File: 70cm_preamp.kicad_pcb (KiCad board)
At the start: 2 copper layers, 33 x 13.2 mm, 10 parts, among them J1 RF_IN, J2 RF_OUT, U1 SF2446E, U2 PGA-103+

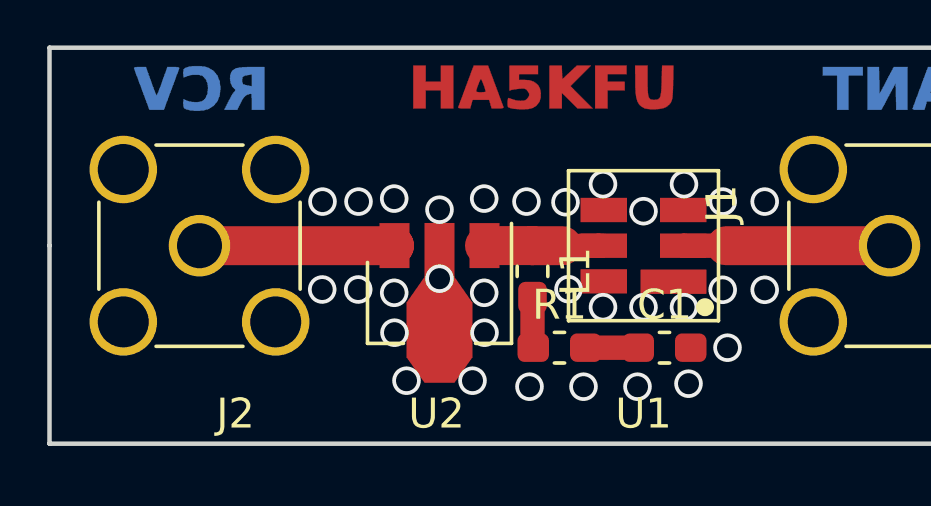
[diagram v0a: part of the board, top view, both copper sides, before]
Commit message: 0805 RLC
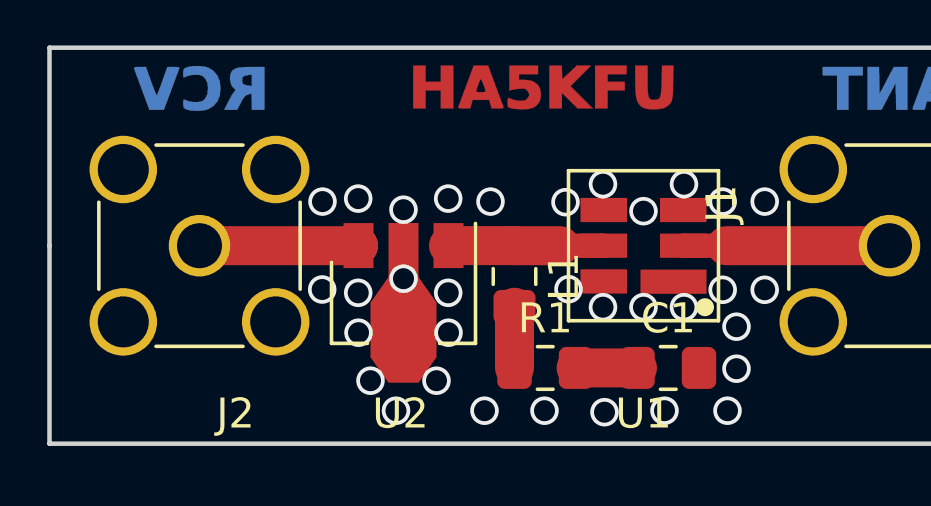
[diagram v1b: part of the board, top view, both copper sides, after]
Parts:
- C1: footprint 70cm_preamp:C_0603_1608Metric_Pad1.05x0.95mm_HandSolder -> 70cm_preamp:C_0805_2012Metric_Pad1.15x1.40mm_HandSolder
- L1: footprint 70cm_preamp:L_0603_1608Metric_Pad1.05x0.95mm_HandSolder -> 70cm_preamp:L_0805_2012Metric_Pad1.15x1.40mm_HandSolder
- R1: footprint 70cm_preamp:R_0603_1608Metric_Pad1.05x0.95mm_HandSolder -> 70cm_preamp:R_0805_2012Metric_Pad1.15x1.40mm_HandSolder
- moved U2 1.20 mm to (54.4, 38.3)
- moved R1 0.83 mm to (59.1, 40.9)
- moved C1 0.69 mm to (63.2, 40.9)
- moved L1 0.62 mm to (58.1, 37.8)
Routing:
- net Net-(L1-Pad1): track 3.38 -> 5.18 mm
- net Net-(J2-Pad1): track 6.50 -> 5.30 mm
- net GND: vias 32 -> 33

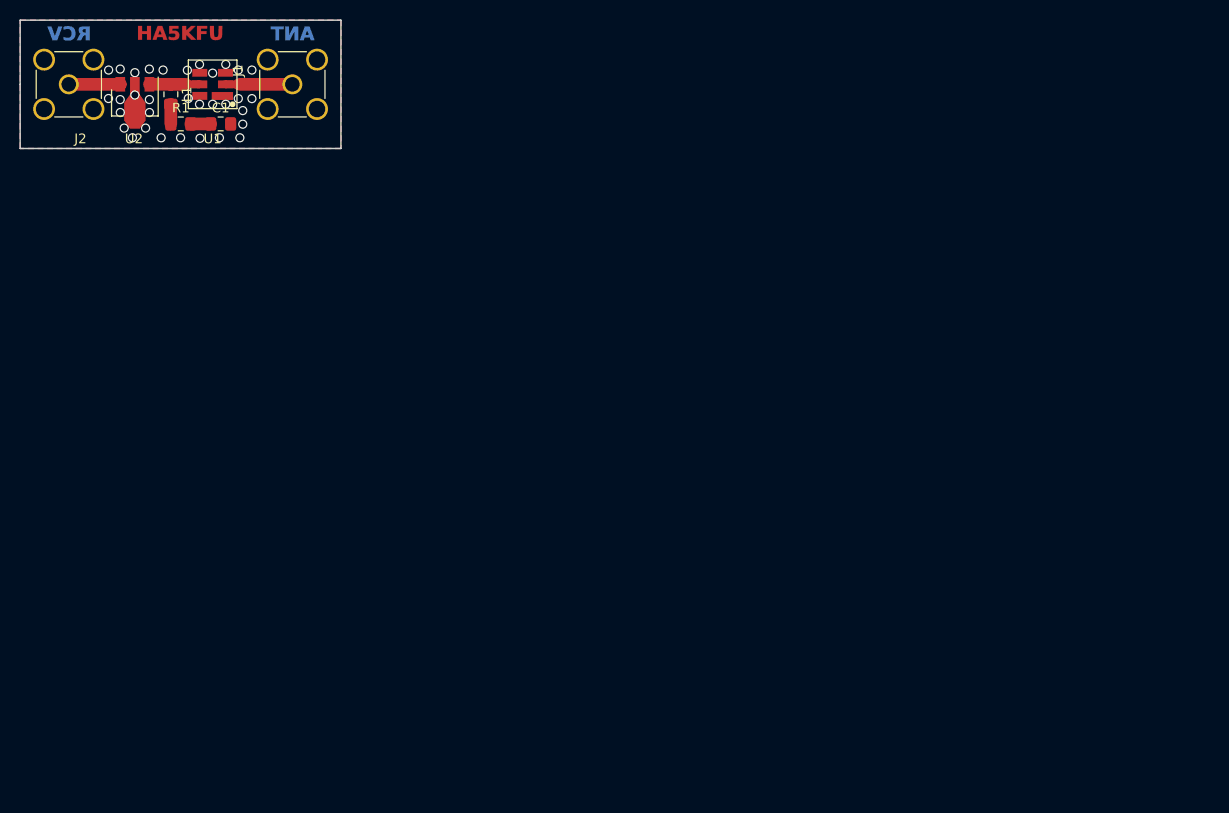
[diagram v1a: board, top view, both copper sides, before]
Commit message: Dokumentáció
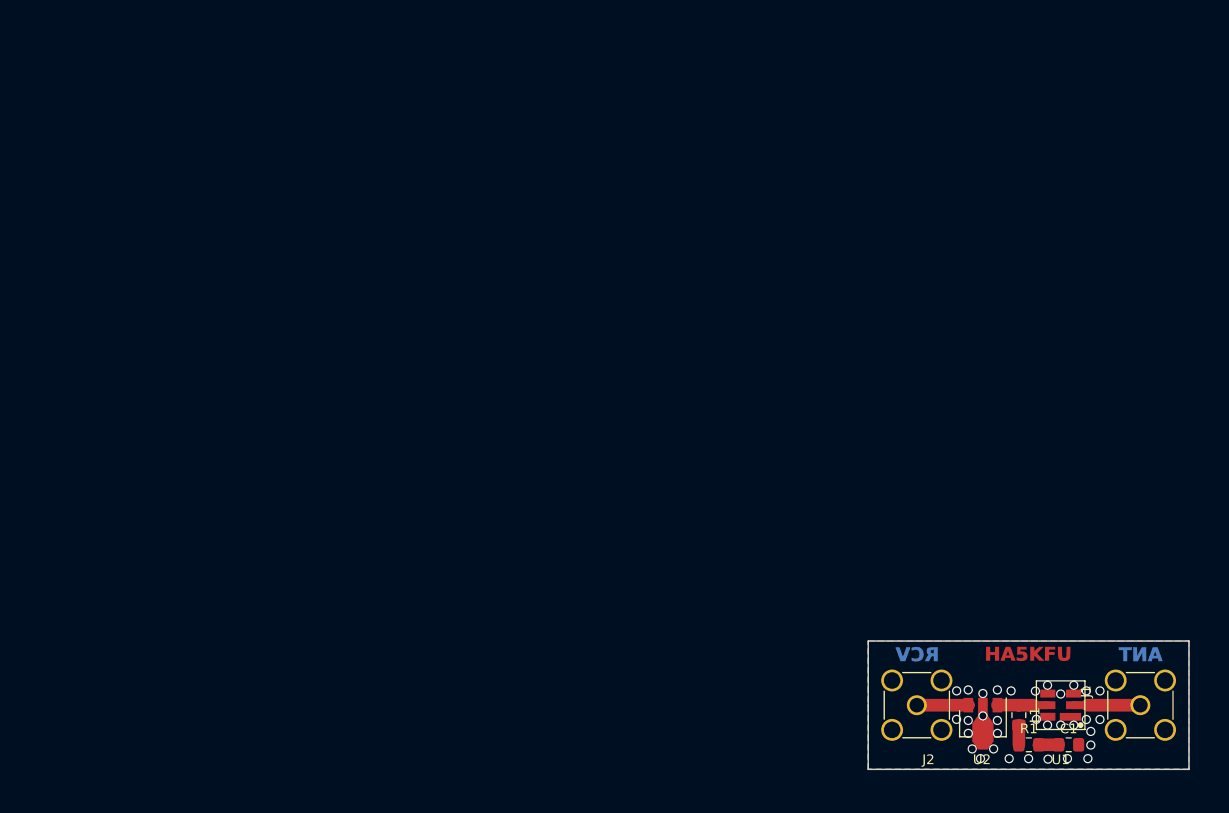
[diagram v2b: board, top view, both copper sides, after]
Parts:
- moved C1 108.1 mm to (150.5, 104.7)
- moved J1 108.1 mm to (157.8, 100.7)
- moved J2 108.1 mm to (134.8, 100.7)
- moved R1 108.1 mm to (146.4, 104.7)
- moved G*** 108.1 mm to (134.8, 95.6)
- moved G*** 108.1 mm to (157.8, 95.6)
- moved G*** 108.1 mm to (146.3, 95.3)
- moved L1 108.1 mm to (145.3, 101.7)
- moved U1 108.1 mm to (149.6, 100.7)
- moved U2 108.1 mm to (141.6, 102.1)

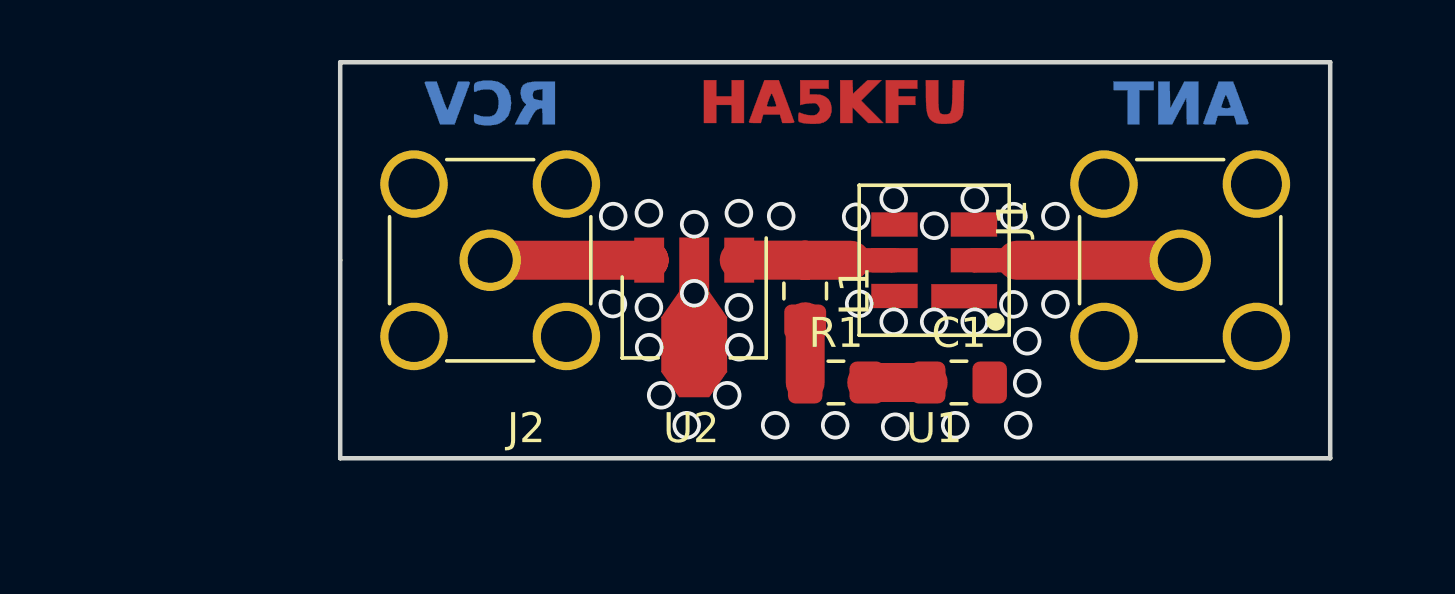
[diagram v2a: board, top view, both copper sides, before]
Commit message: Add a few parts
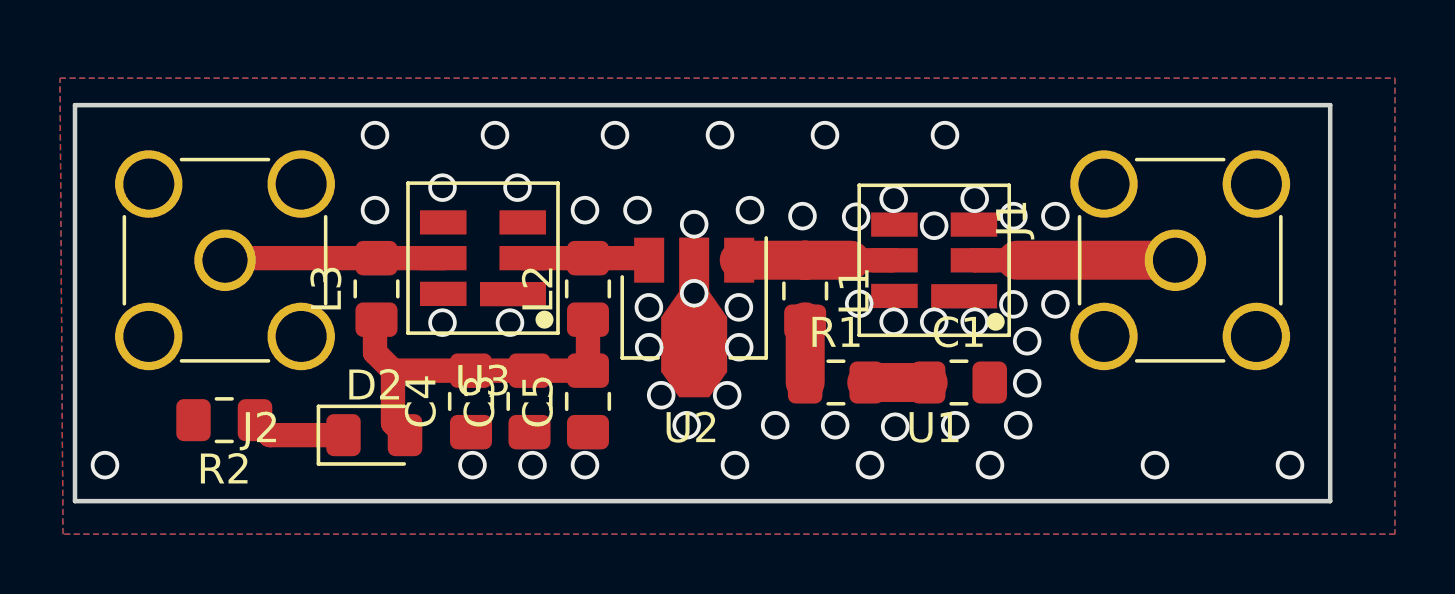
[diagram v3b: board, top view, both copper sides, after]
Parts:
- removed G***: LOGO, 70cm_preamp:RCV
- removed G***: LOGO, 70cm_preamp:ANT
- removed G***: LOGO, 70cm_preamp:HA5KFU
- added C3: 330p, 70cm_preamp:C_0805_2012Metric_Pad1.15x1.40mm_HandSolder, F.Cu at (136.2, 105.4)
- added C4: 330p, 70cm_preamp:C_0805_2012Metric_Pad1.15x1.40mm_HandSolder, F.Cu at (134.2, 105.4)
- added C5: 330p, 70cm_preamp:C_0805_2012Metric_Pad1.15x1.40mm_HandSolder, F.Cu at (138.1, 105.4)
- added D2: LED, LED_SMD:LED_0805_2012Metric_Pad1.15x1.40mm_HandSolder, F.Cu at (131.0, 106.5)
- added L2: 620n, 70cm_preamp:L_0805_2012Metric_Pad1.15x1.40mm_HandSolder, F.Cu at (138.1, 101.6)
- added L3: 620n, 70cm_preamp:L_0805_2012Metric_Pad1.15x1.40mm_HandSolder, F.Cu at (131.1, 101.6)
- added R2: 330, 70cm_preamp:R_0805_2012Metric_Pad1.15x1.40mm_HandSolder, F.Cu at (126.0, 106.0)
- added U3: SF2446E, 70cm_preamp:SF2446E-Filter_Custom_HandSolder, F.Cu at (134.6, 100.6)
- moved J2 8.84 mm to (126.0, 100.7)
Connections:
- J2 pad 1: Net-(J2-Pad1) -> Net-(J2-In)
- U2 pad 3: Net-(J2-Pad1) -> Net-(JP1-A)
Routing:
- net Net-(D2-A): track 0.00 -> 12.5 mm
- net Net-(J2-In): track 0.00 -> 7.30 mm
- net Net-(J2-Pad1): track 5.30 -> 0.00 mm
- net Net-(JP1-A): track 0.00 -> 4.24 mm
- net Net-(D2-K): track 0.00 -> 3.16 mm
- net GND: vias 33 -> 52
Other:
- board size 33 x 13.2 mm -> 41.8 x 13.2 mm
- net class Default removed
- net class Tapvonal_vastag removed
- net class Tapvonal_vekony removed
- board text added: "HA5KFU HA8KDA 2023 MRC-100"
- board text added: "PWR"
